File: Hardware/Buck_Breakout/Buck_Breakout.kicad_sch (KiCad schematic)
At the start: 9 parts, among them U1 AP62200WU

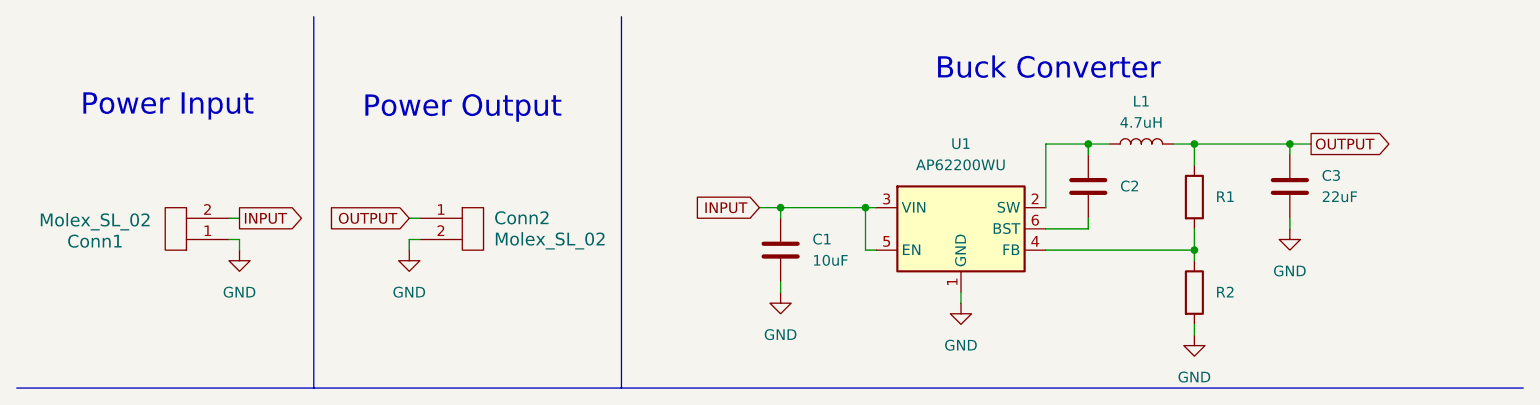
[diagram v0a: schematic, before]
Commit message: Generate BOM for buck breakout
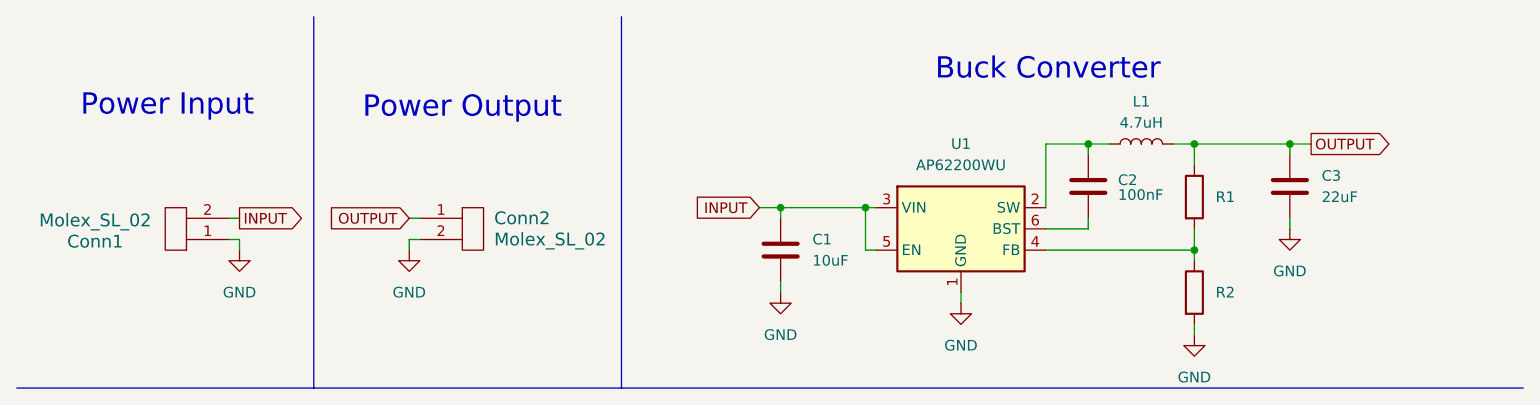
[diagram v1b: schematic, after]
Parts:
- C2: value C -> 100nF
- R1: value R -> R1
- R2: value R -> R2
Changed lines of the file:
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@@
 			)
 		)
-		(property "Value" "R"
+		(property "Value" "R2"
 			(at 154.94 45.7199 0)
 			(effects
@@
 		(on_board yes)
 		(dnp no)
-		(fields_autoplaced yes)
 		(property "Reference" "C2"
-			(at 143.51 31.7499 0)
-			(effects
-				(font
-					(size 1.27 1.27)
-				)
-				(justify left)
-			)
-		)
-		(property "Value" "C"
-			(at 143.51 33.0199 0)
-			(effects
-				(font
-					(size 1.27 1.27)
-				)
-				(justify left)
-				(hide yes)
+			(at 143.256 30.9879 0)
+			(effects
+				(font
+					(size 1.27 1.27)
+				)
+				(justify left)
+			)
+		)
+		(property "Value" "100nF"
+			(at 143.256 32.766 0)
+			(effects
+				(font
+					(size 1.27 1.27)
+				)
+				(justify left)
 			)
 		)
@@
 			)
 		)
-		(property "Value" "R"
+		(property "Value" "R1"
 			(at 154.94 34.2899 0)
 			(effects
